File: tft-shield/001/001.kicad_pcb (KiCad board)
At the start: 2 copper layers, 28.6 x 17.8 mm, 7 parts, among them J1 CONN_01X08, Q1 S8050, U1 TFT_0.9680*160

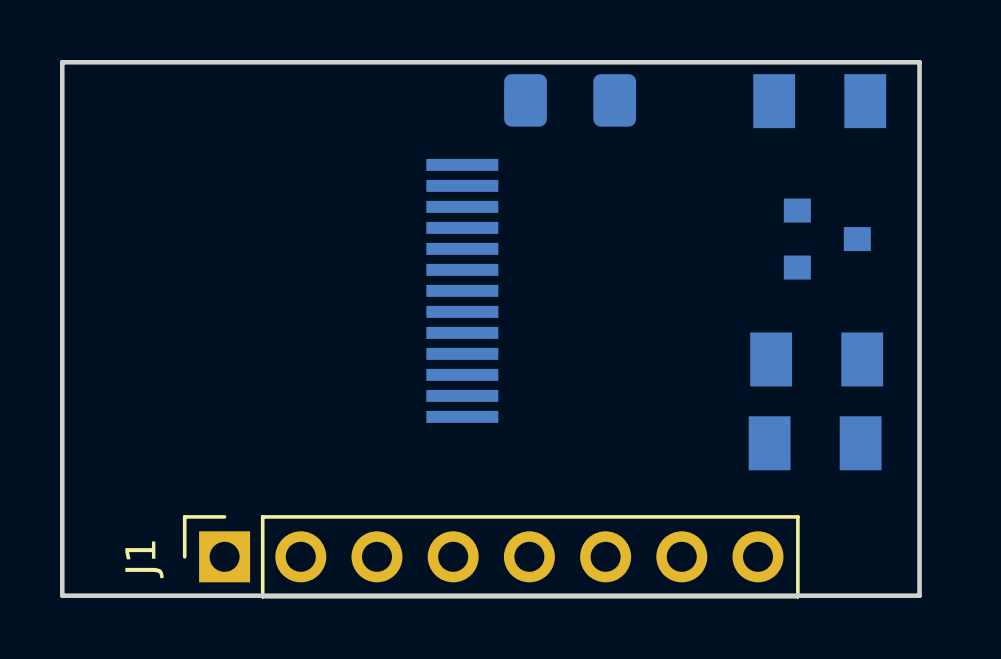
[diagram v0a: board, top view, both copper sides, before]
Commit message: Add some changess & 3d model
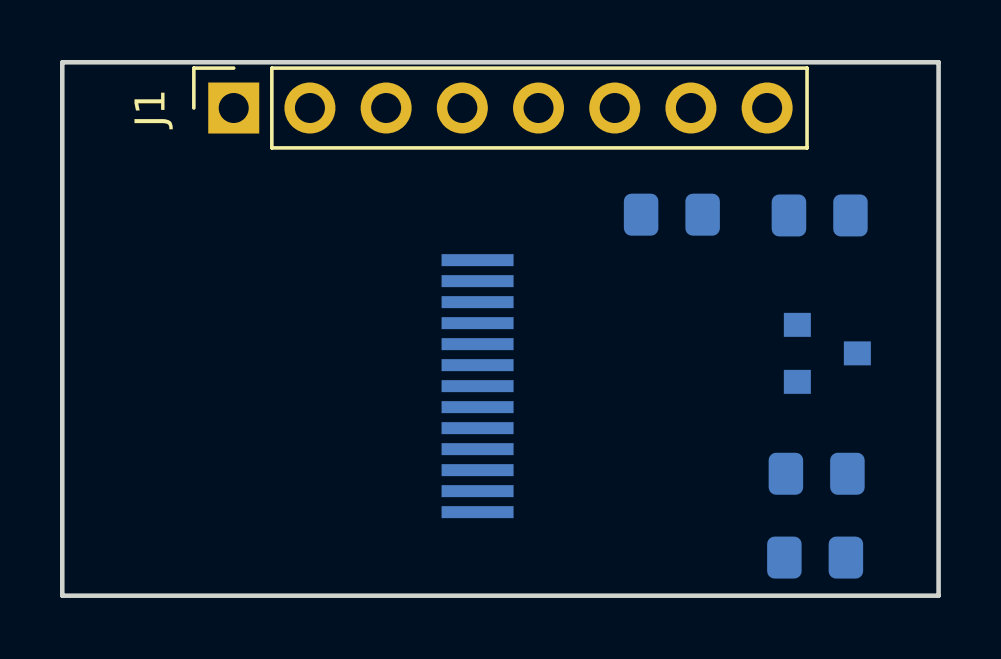
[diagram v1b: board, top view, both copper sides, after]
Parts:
- C1: footprint Capacitor_SMD:C_1206_3216Metric_Pad1.42x1.75mm_HandSolder -> Capacitor_SMD:C_0805_2012Metric_Pad1.15x1.40mm_HandSolder
- R1, R2, R3: footprint Resistor_SMD:R_1206_3216Metric_Pad1.39x1.80mm_HandSolder -> Resistor_SMD:R_0805_2012Metric_Pad1.15x1.40mm_HandSolder
- moved J1 15.0 mm to (130.2, 83.4)
- moved C1 5.10 mm to (144.8, 87.0)
- moved Q1 3.81 mm to (150.0, 91.6)
- moved R1 3.81 mm to (149.6, 95.6)
- moved R2 3.81 mm to (149.6, 98.4)
- moved R3 3.81 mm to (149.7, 87.0)
- moved U1 3.22 mm to (138.3, 92.7)
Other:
- board size 28.6 x 17.8 mm -> 29.2 x 17.8 mm
